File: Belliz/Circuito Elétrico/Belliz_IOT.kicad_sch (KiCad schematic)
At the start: 24 parts, among them J1 Conector MAX6675, J2 Conector TCRT5000, J3 Conector ACS712, J4 440054-2, J5 Conn_01x10_Socket, J6 Conector P4, J7 KK_2vias, J8 440054-2, U1 ESP32-WROOM-32D, U2 LM358, U3 LM358

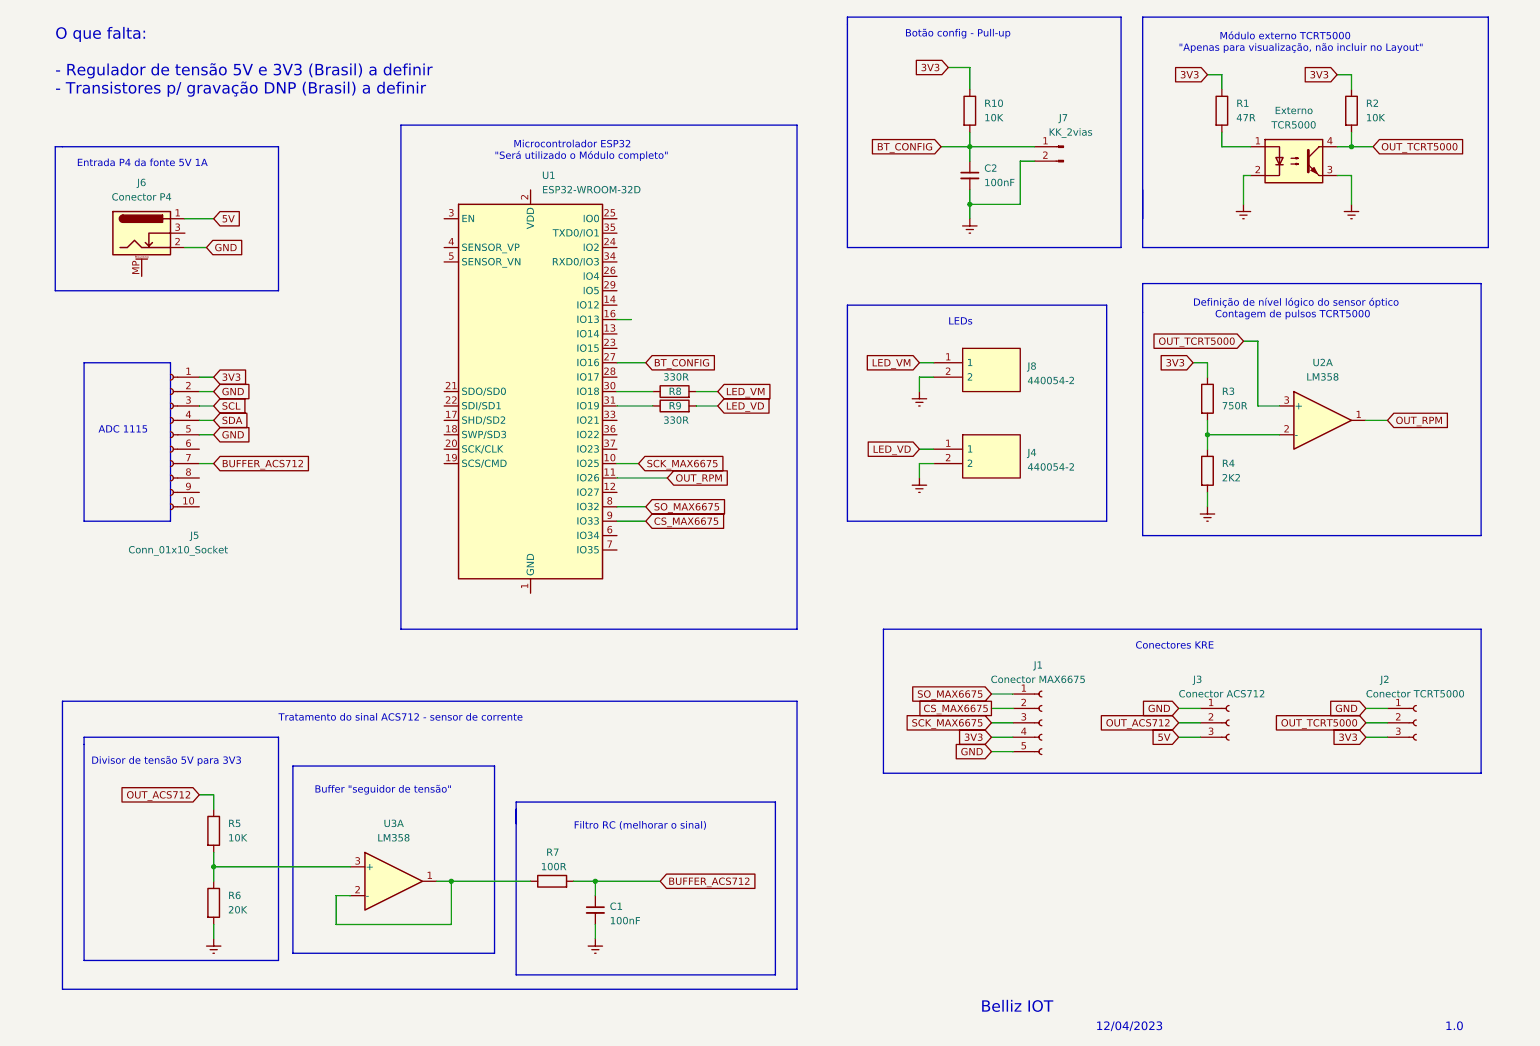
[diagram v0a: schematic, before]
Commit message: Inclusao da pasta do fw
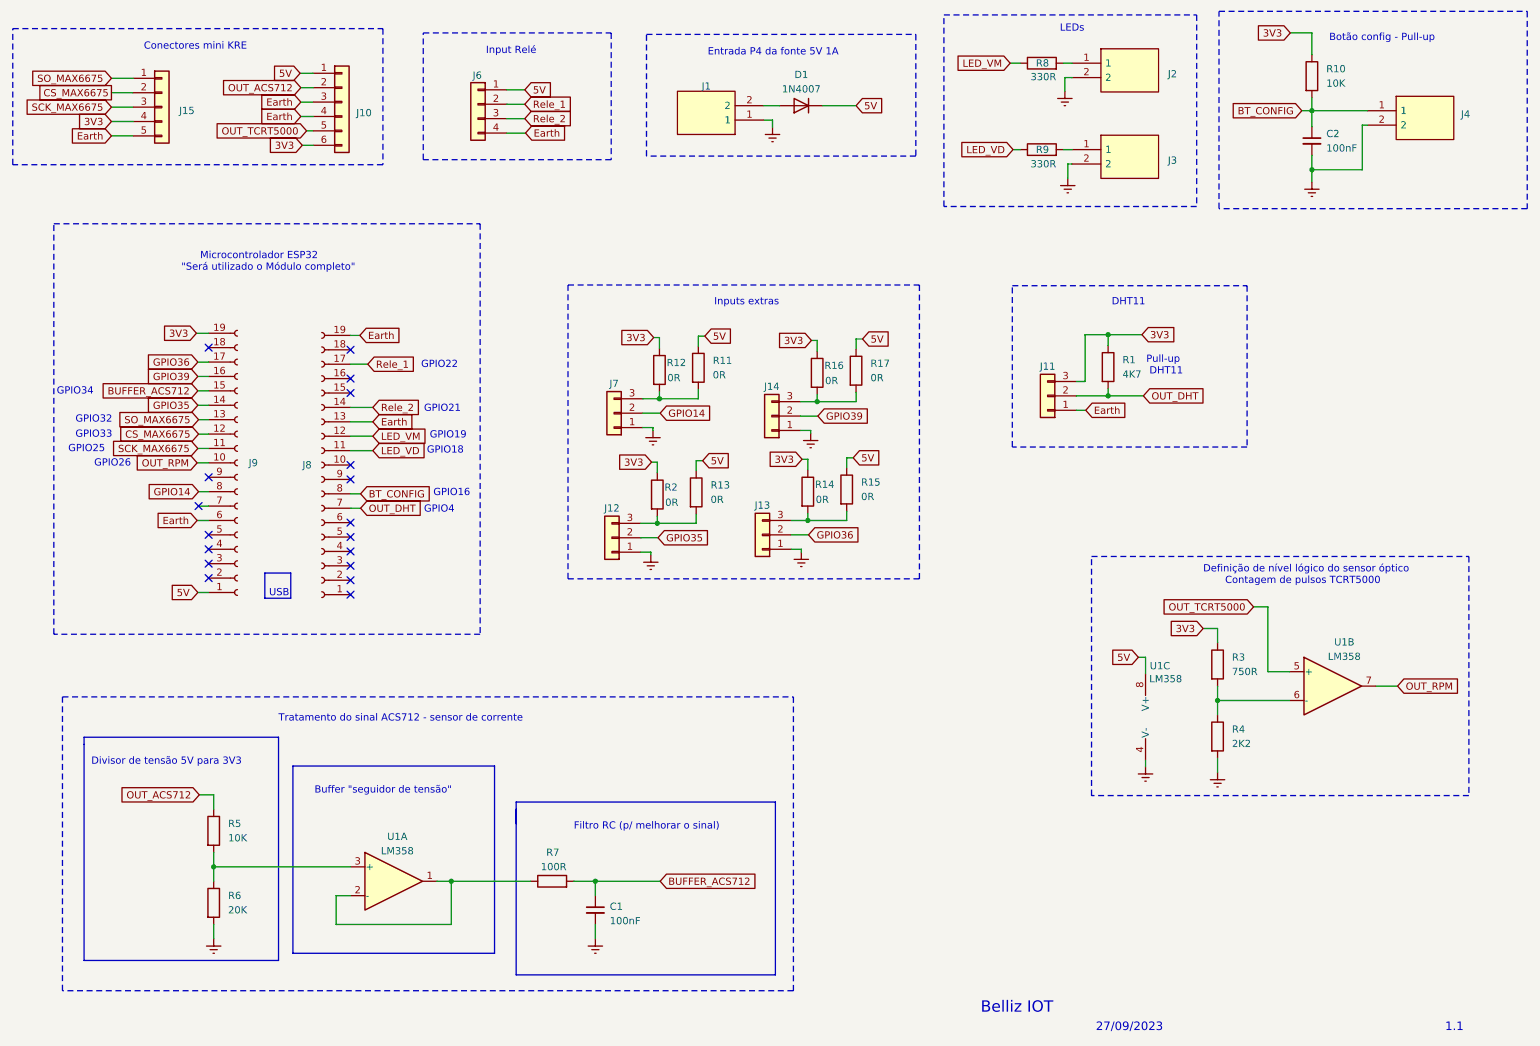
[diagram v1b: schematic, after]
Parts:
- removed Externo: TCR5000, Package_SO:SOP-4_4.4x2.6mm_P1.27mm, symbol Isolator:FODM217B
- removed J1: Conector MAX6675, symbol Connector:Conn_01x05_Female
- removed J2: Conector TCRT5000, symbol Connector:Conn_01x03_Female
- removed J3: Conector ACS712, symbol Connector:Conn_01x03_Female
- removed J5: Conn_01x10_Socket, symbol Connector:Conn_01x10_Socket
- removed J6: Conector P4, symbol Connector:Barrel_Jack_Switch_MountingPin
- removed J7: KK_2vias, symbol Connector:Conn_01x02_Male
- removed U1: ESP32-WROOM-32D, RF_Module:ESP32-WROOM-32, symbol RF_Module:ESP32-WROOM-32D
- added D1: 1N4007, Diode_THT:D_DO-41_SOD81_P10.16mm_Horizontal, symbol Diode:1N4007
- added J1: ~, My_library_footprint:KK_2vias, symbol My_library:440054-2
- added J10: Conn_01x06, My_library_footprint:KRE_6Vias, symbol Connector_Generic:Conn_01x06
- added J11, J12, J13, J14, J7: Conn_01x03, My_library_footprint:KK_3Vias, symbol Connector_Generic:Conn_01x03
- added J15: Conn_01x05, My_library_footprint:KRE_5Vias, symbol Connector_Generic:Conn_01x05
- added J4: 440054-2, My_library_footprint:KK_2vias, symbol My_library:440054-2
- added J6: Conn_01x04, My_library_footprint:KK_4vias, symbol Connector_Generic:Conn_01x04
- added J8, J9: Conn_01x19_Socket, My_library_footprint:Pin_header_19vias_female, symbol Connector:Conn_01x19_Socket
- added R11, R12, R13, R14, R15, R16, R17: 0R, Resistor_SMD:R_0805_2012Metric, symbol Device:R
- added unit 3 of U1
- C1, C2: footprint (none) -> Capacitor_SMD:C_0805_2012Metric
- J2: renamed from J8; footprint My_library_footprint:440054-2 -> My_library_footprint:KK_2vias
- J3: renamed from J4; footprint My_library_footprint:440054-2 -> My_library_footprint:KK_2vias
- R1: value 47R -> 4K7; footprint (none) -> Resistor_SMD:R_0805_2012Metric
- R10, R3, R4, R5, R6, R7, R8, R9: footprint (none) -> Resistor_SMD:R_0805_2012Metric
- R2: value 10K -> 0R; footprint (none) -> Resistor_SMD:R_0805_2012Metric
- U1: renamed from U2; footprint (none) -> Package_DIP:DIP-8_W7.62mm
- U1: renamed from U3; footprint (none) -> Package_DIP:DIP-8_W7.62mm
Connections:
- net 3V3: now also J10.6 (Pin_6), J11.3 (Pin_3), J15.4 (Pin_4), J9.19 (Pin_19), R12.1, R14.1, R16.1
- net 5V: now also D1.1 (K), J10.1 (Pin_1), J6.1 (Pin_1), J9.1 (Pin_1), R11.1, R13.1, R15.1, R17.1, U1.8 (V+)
- net BT_CONFIG: now also J4.1, J8.8 (Pin_8)
- net BUFFER_ACS712: now also J9.15 (Pin_15)
- net CS_MAX6675: now also J15.2 (Pin_2), J9.12 (Pin_12)
- net Earth: now also J1.1, J10.3 (Pin_3), J10.4 (Pin_4), J11.1 (Pin_1), J12.1 (Pin_1), J13.1 (Pin_1), J14.1 (Pin_1), J15.5 (Pin_5), J4.2, J6.4 (Pin_4), J7.1 (Pin_1), J8.13 (Pin_13), J8.19 (Pin_19), J9.6 (Pin_6), U1.4 (V-)
- net LED_VD: now also R9.1, J8.11 (Pin_11); no longer J3.1, R9.2
- net LED_VM: now also R8.1, J8.12 (Pin_12); no longer J2.1, R8.2
- net OUT_ACS712: now also J10.2 (Pin_2)
- net OUT_RPM: now also U1.7, J9.10 (Pin_10); no longer U1.1
- net OUT_TCRT5000: now also U1.5 (+), J10.5 (Pin_5); no longer R2.2, U1.3 (+)
- net SCK_MAX6675: now also J15.3 (Pin_3), J9.11 (Pin_11)
- net SO_MAX6675: now also J15.1 (Pin_1), J9.13 (Pin_13)
- net OUT_DHT: now reaches R1.2
- net OUT_DHT: now also J11.2 (Pin_2), J8.7 (Pin_7)
- net at R3.2, R4.1: now also U1.6 (-); no longer U1.2 (-)
- new net: J7.3 (Pin_3), R11.2, R12.2
- new net: J3.1, R9.2
- new net: J12.3 (Pin_3), R13.2, R2.2
- new net: J14.3 (Pin_3), R16.2, R17.2
- new net: D1.2 (A), J1.2
- new net: J2.1, R8.2
- new net: J13.3 (Pin_3), R14.2, R15.2
- new net GPIO14: J7.2 (Pin_2), J9.8 (Pin_8)
- new net GPIO35: J12.2 (Pin_2), J9.14 (Pin_14)
- new net GPIO36: J13.2 (Pin_2), J9.17 (Pin_17)
- new net GPIO39: J14.2 (Pin_2), J9.16 (Pin_16)
- new net Rele_1: J6.2 (Pin_2), J8.17 (Pin_17)
- new net Rele_2: J6.3 (Pin_3), J8.14 (Pin_14)
- no-connect marks 0 -> 18
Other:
- note added: "1.1"
- note added: "27/09/2023"
- note added: "Conectores mini KRE"
- note added: "DHT11"
- note added: "Filtro RC (p/ melhorar o sinal)"
- note added: "GPIO16"
- note added: "GPIO18"
- note added: "GPIO19"
- note added: "GPIO21"
- note added: "GPIO22"
- note added: "GPIO25"
- note added: "GPIO26"
- note added: "GPIO32"
- note added: "GPIO33"
- note added: "GPIO34"
- note added: "GPIO4"
- note added: "Input Relé"
- note added: "Inputs extras"
- note added: "Pull-up DHT11"
- note added: "USB"
- note removed: "1.0"
- note removed: "12/04/2023"
- note removed: "ADC 1115"
- note removed: "Conectores KRE"
- note removed: "Filtro RC (melhorar o sinal)"
- note removed: "Módulo externo TCRT5000 "Apenas para visualização, não incluir no Layout""
- note removed: "O que falta: - Regulador de tensão 5V e 3V3 (Brasil) a definir - Transistores p/ gravação DNP (Brasil) a definir"
- moved on the sheet: C2, J2, J3, R10, R3, R4, R8, R9, U1B

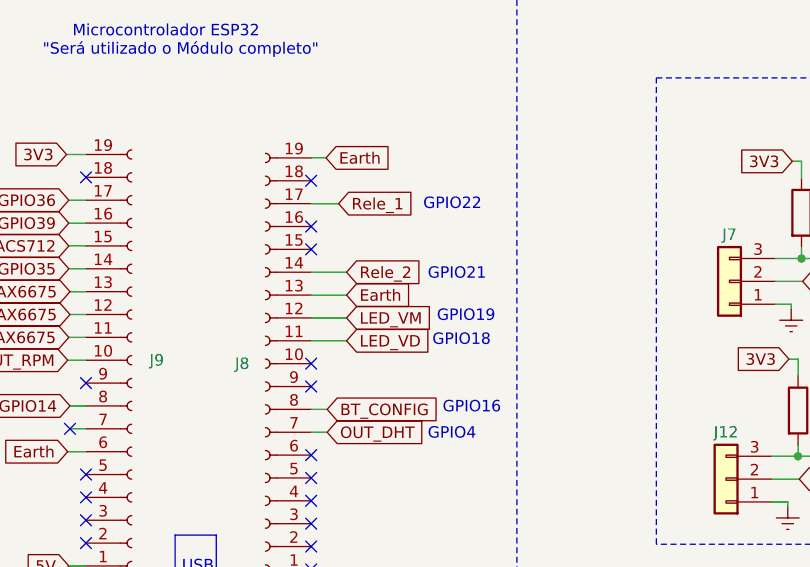
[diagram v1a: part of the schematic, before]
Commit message: código funcional
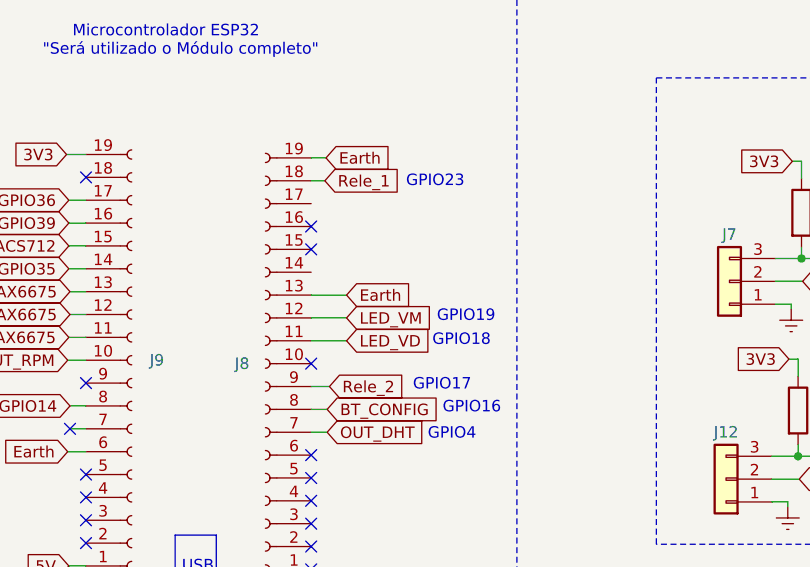
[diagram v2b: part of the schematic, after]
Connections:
- net Rele_1: now also J8.18 (Pin_18); no longer J8.17 (Pin_17)
- net Rele_2: now also J8.9 (Pin_9); no longer J8.14 (Pin_14)
- no-connect marks 18 -> 16
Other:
- note added: "GPIO17"
- note added: "GPIO23"
- note removed: "GPIO21"
- note removed: "GPIO22"
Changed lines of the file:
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@@
   (no_connect (at 49.911 114.173))
   (no_connect (at 48.133 101.473))
-  (no_connect (at 74.93 73.914))
   (no_connect (at 49.911 73.533))
   (no_connect (at 49.911 111.633))
@@
   (no_connect (at 49.911 106.553))
   (no_connect (at 74.93 117.094))
-  (no_connect (at 74.93 96.774))
   (no_connect (at 49.911 96.393))
   (wire (pts (xy 36.576 36.195) (xy 32.766 36.195))
@@
     (stroke (width 0) (type default))
   )
-  (wire (pts (xy 74.93 76.454) (xy 77.978 76.454))
-    (stroke (width 0) (type default))
-  )
   (wire (pts (xy 102.489 35.687) (xy 105.791 35.687))
     (stroke (width 0) (type default))
@@
     (stroke (width 0) (type default))
   )
-  (wire (pts (xy 74.93 84.074) (xy 78.867 84.074))
-    (stroke (width 0) (type default))
-  )
   (wire (pts (xy 49.911 88.773) (xy 48.133 88.773))
     (stroke (width 0) (type default))
@@
     (stroke (width 0) (type default))
   )
+  (wire (pts (xy 74.93 96.774) (xy 76.962 96.774))
+    (stroke (width 0) (type default))
+  )
   (wire (pts (xy 128.016 93.726) (xy 129.032 93.726))
     (stroke (width 0) (type default))
@@
   )
   (wire (pts (xy 66.167 30.226) (xy 68.326 30.226))
+    (stroke (width 0) (type default))
+  )
+  (wire (pts (xy 74.93 73.914) (xy 76.454 73.914))
     (stroke (width 0) (type default))
   )
@@
     (effects (font (size 1.27 1.27)) (justify left bottom))
   )
+  (text "GPIO23\n\n" (at 85.471 76.835 0)
+    (effects (font (size 1.27 1.27)) (justify left bottom))
+  )
   (text "      Microcontrolador ESP32 \n\"Será utilizado o Módulo completo\""
     (at 45.085 60.198 0)
@@
     (effects (font (size 1.27 1.27)) (justify left bottom))
   )
-  (text "GPIO22\n" (at 87.376 77.343 0)
-    (effects (font (size 1.27 1.27)) (justify left bottom))
-  )
   (text "Filtro RC (p/ melhorar o sinal)" (at 114.3 158.75 0)
     (effects (font (size 1.27 1.27)) (justify left bottom))
@@
     (effects (font (size 2 2)) (justify left bottom))
   )
+  (text "GPIO17\n\n" (at 86.233 99.441 0)
+    (effects (font (size 1.27 1.27)) (justify left bottom))
+  )
   (text "Pull-up \n DHT11" (at 215.265 78.486 0)
     (effects (font (size 1.27 1.27)) (justify left bottom))
@@
     (effects (font (size 1.27 1.27)) (justify left bottom))
   )
-  (text "GPIO21\n" (at 87.884 85.09 0)
-    (effects (font (size 1.27 1.27)) (justify left bottom))
-  )
   (text "Botão config - Pull-up" (at 247.523 19.685 0)
     (effects (font (size 1.27 1.27)) (justify left bottom))
@@
     )
   )
-  (global_label "Rele_2" (shape input) (at 78.867 84.074 0) (fields_autoplaced)
-    (effects (font (size 1.27 1.27)) (justify left))
-    (property "Intersheetrefs" "${INTERSHEET_REFS}" (at 88.0623 84.074 0)
-      (effects (font (size 1.27 1.27)) (justify left) hide)
-    )
-  )
-  (global_label "Rele_1" (shape input) (at 77.978 76.454 0) (fields_autoplaced)
-    (effects (font (size 1.27 1.27)) (justify left))
-    (property "Intersheetrefs" "${INTERSHEET_REFS}" (at 87.1733 76.454 0)
-      (effects (font (size 1.27 1.27)) (justify left) hide)
-    )
+  (global_label "Rele_2" (shape input) (at 76.962 96.774 0) (fields_autoplaced)
+    (effects (font (size 1.27 1.27)) (justify left))
+    (property "Intersheetrefs" "${INTERSHEET_REFS}" (at 86.1573 96.774 0)
+      (effects (font (size 1.27 1.27)) (justify left) hide)
+    )
+  )
+  (global_label "Rele_1" (shape input) (at 76.454 73.914 0) (fields_autoplaced)
+    (effects (font (size 1.27 1.27)) (justify left))
+    (property "Intersheetrefs" "${INTERSHEET_REFS}" (at 85.6493 73.914 0)
+      (effects (font (size 1.27 1.27)) (justify left) hide)
+    )
